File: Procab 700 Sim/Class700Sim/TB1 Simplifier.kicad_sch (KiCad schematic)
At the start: 0 parts

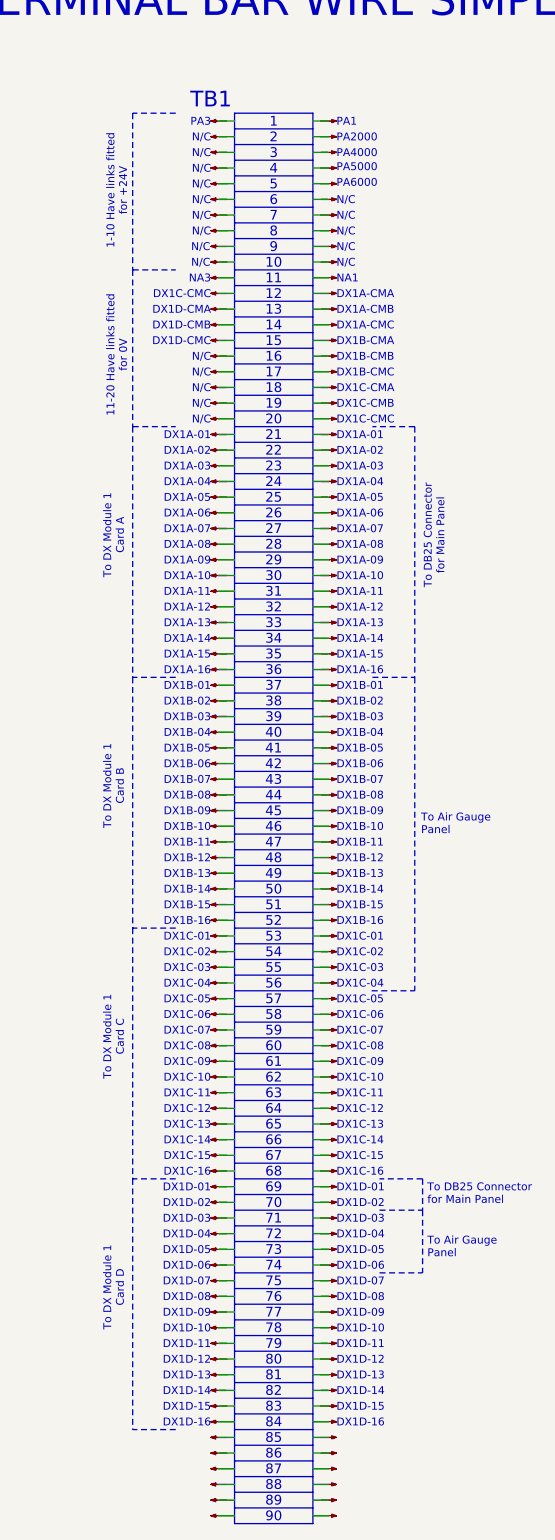
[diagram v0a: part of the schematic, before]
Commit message: TB2 added
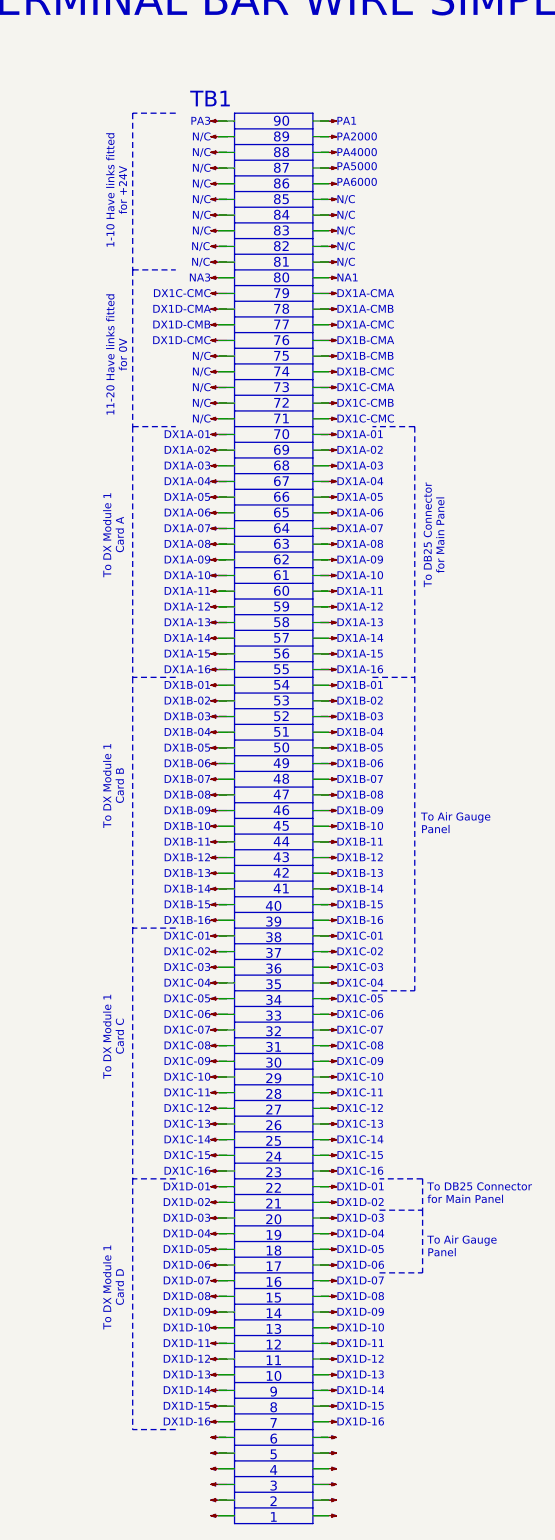
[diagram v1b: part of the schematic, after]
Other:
- note added: "40 39 38 37 36 35 34 33 32 31 30 29 28 27 26 25 24 23 22 21 20 19 18 17 16 15 14 13 12 11 10 9 8 7 6 5 4 3 2 1"
- note added: "90 89 88 87 86 85 84 83 82 81 80 79 78 77 76 75 74 73 72 71 70 69 68 67 66 65 64 63 62 61 60 59 58 57 56 55 54 53 52 51 50 49 48 47 46 45 44 43 42 41"
- note removed: "1 2 3 4 5 6 7 8 9 10 11 12 13 14 15 16 17 18 19 20 21 22 23 24 25 26 27 28 29 30 31 32 33 34 35 36 37 38 39 40"
- note removed: "41 42 43 44 45 46 47 48 49 50 51 52 53 54 55 56 57 58 59 60 61 62 63 64 65 66 67 68 69 70 71 72 73 74 75 76 77 78 79 80 81 82 83 84 85 86 87 88 89 90"
